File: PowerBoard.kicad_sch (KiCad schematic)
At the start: 30 parts, among them Q1 Q_NMOS_GDS, Q2 Q_PMOS_GDS, Q3 Q_PMOS_GDS, SW5 SW_SPDT, U10 MT2492, U11 MT2492

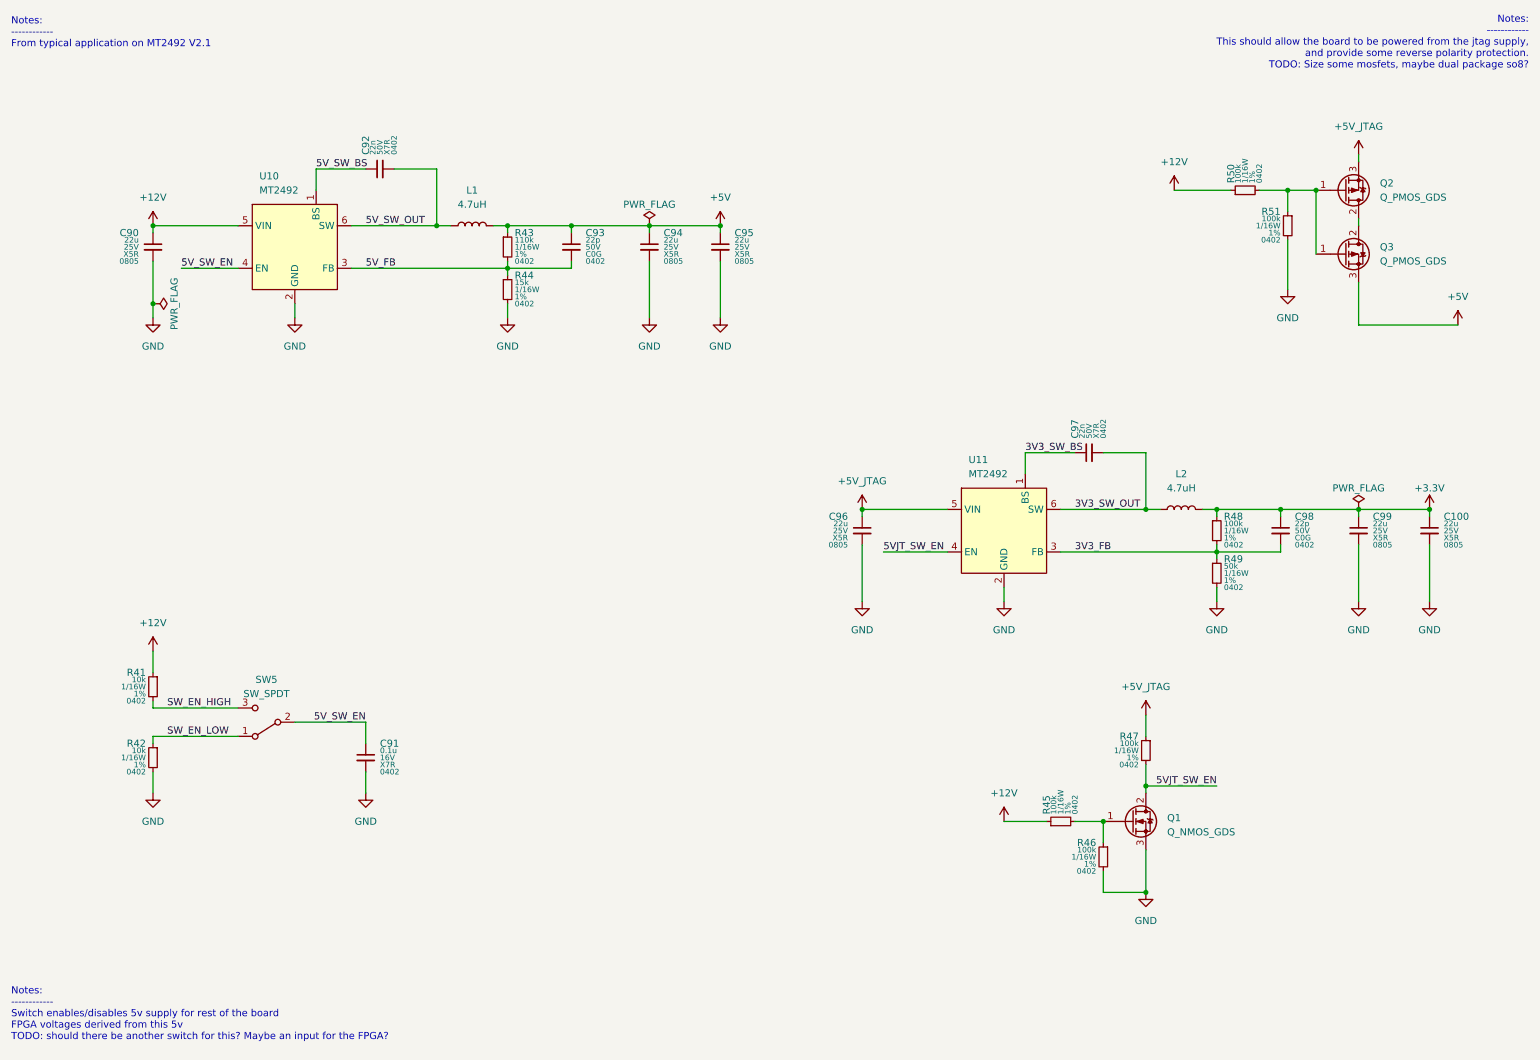
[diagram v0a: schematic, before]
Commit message: Second pass
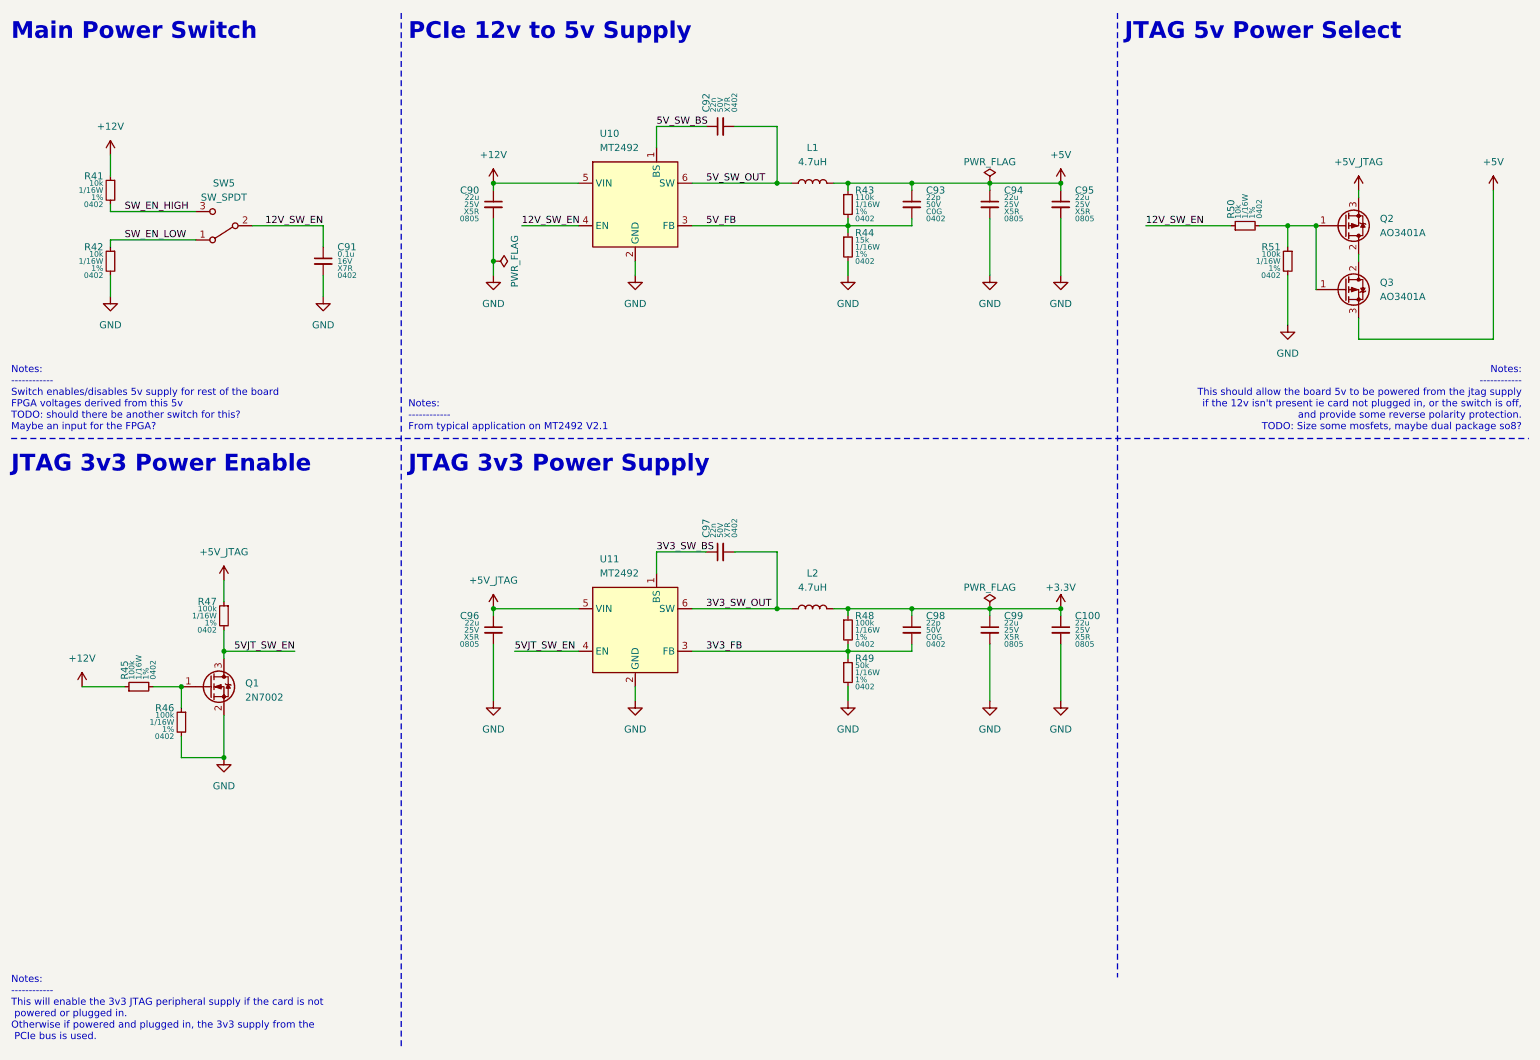
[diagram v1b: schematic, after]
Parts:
- removed Q1: Q_NMOS_GDS, Package_TO_SOT_SMD:SOT-23, symbol Device:Q_NMOS_GDS
- added Q1: 2N7002, Package_TO_SOT_SMD:SOT-23, symbol Transistor_FET:2N7002
- Q2, Q3: value Q_PMOS_GDS -> AO3401A
- R50: value 100k -> 10k
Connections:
- net +12V: no longer R50.1
- net 5VJT_SW_EN: now also Q1.3 (D)
- net GND: now also Q1.2 (S)
- net at R45.2, R46.1: now also Q1.1 (G)
- net 5V_SW_EN renamed 12V_SW_EN
- net 12V_SW_EN: now also R50.1
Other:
- note added: "JTAG 3v3 Power Enable"
- note added: "JTAG 3v3 Power Supply"
- note added: "JTAG 5v Power Select"
- note added: "Main Power Switch"
- note added: "Notes: ------------ This should allow the board 5v to be powered from the jtag supply if the 12v isn't present ie card not plugged in, or the switch is off, and provide some reverse polarity protection. TODO: Size some mosfets, maybe dual package so8?"
- note added: "Notes: ------------ This will enable the 3v3 JTAG peripheral supply if the card is not powered or plugged in. Otherwise if powered and plugged in, the 3v3 supply from the PCIe bus is used."
- note added: "PCIe 12v to 5v Supply"
- note removed: "Notes: ------------ This should allow the board to be powered from the jtag supply, and provide some reverse polarity protection. TODO: Size some mosfets, maybe dual package so8?"
- moved on the sheet: C100, C90, C91, C92, C93, C94, C95, C96, C97, C98, C99, L1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
